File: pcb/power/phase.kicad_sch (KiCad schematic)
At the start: 9 parts, among them J1 Conn_01x02_Pin, J4 Conn_01x02_Pin, J7 Conn_01x02_Pin, Q10 IPT015N10NF2S, Q2 IPT015N10NF2S, Q5 IPT015N10NF2S, Q6 IPT015N10NF2S

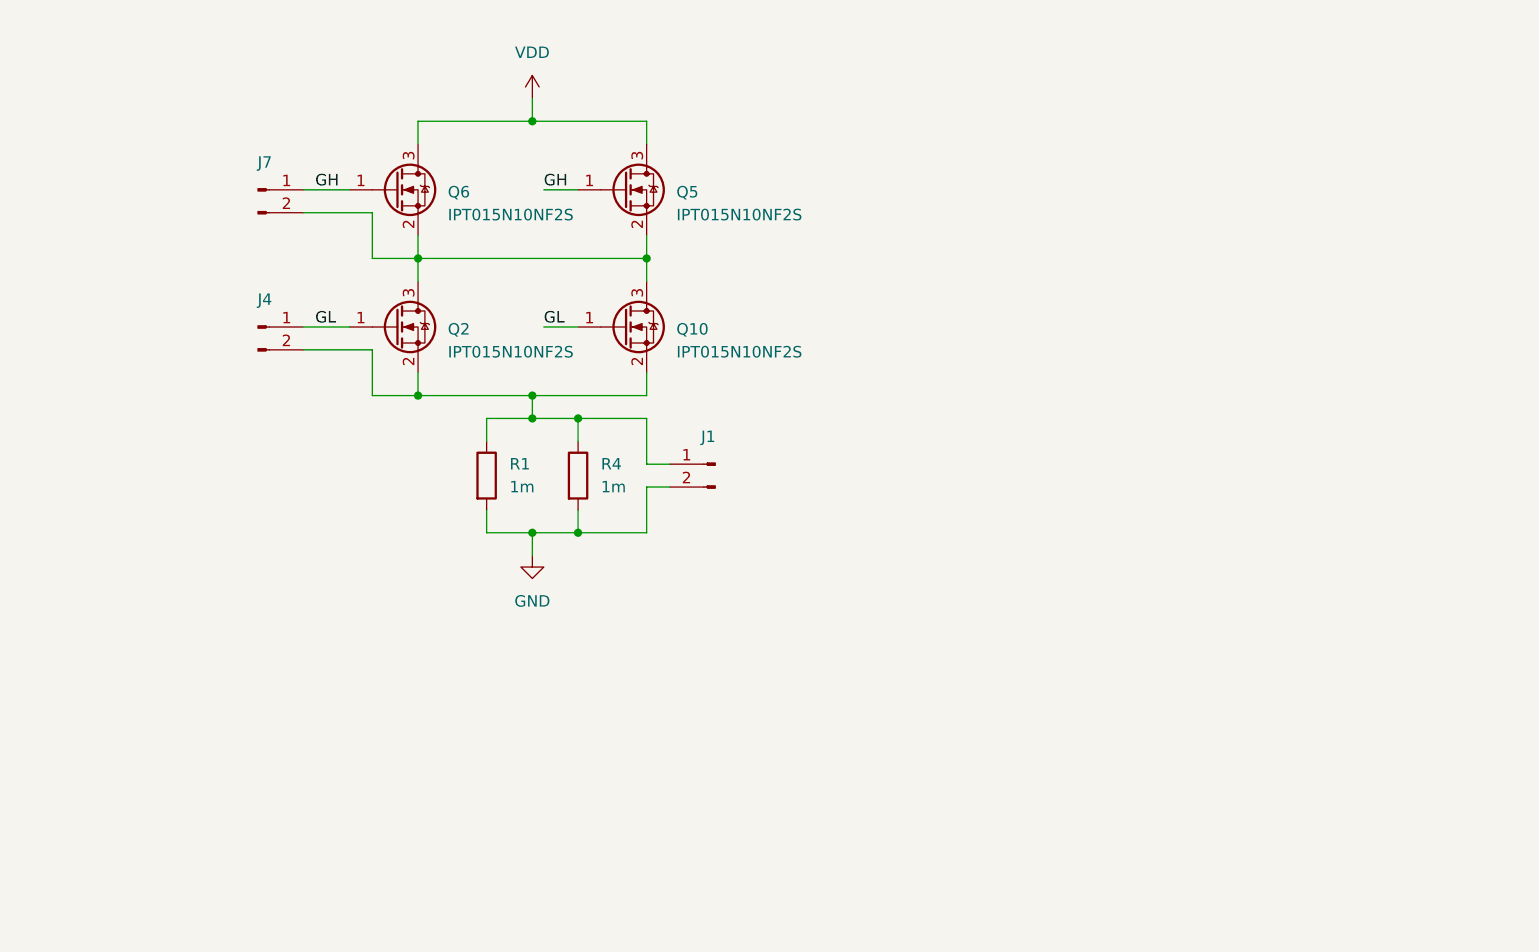
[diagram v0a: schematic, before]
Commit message: Semifinish power and bulk
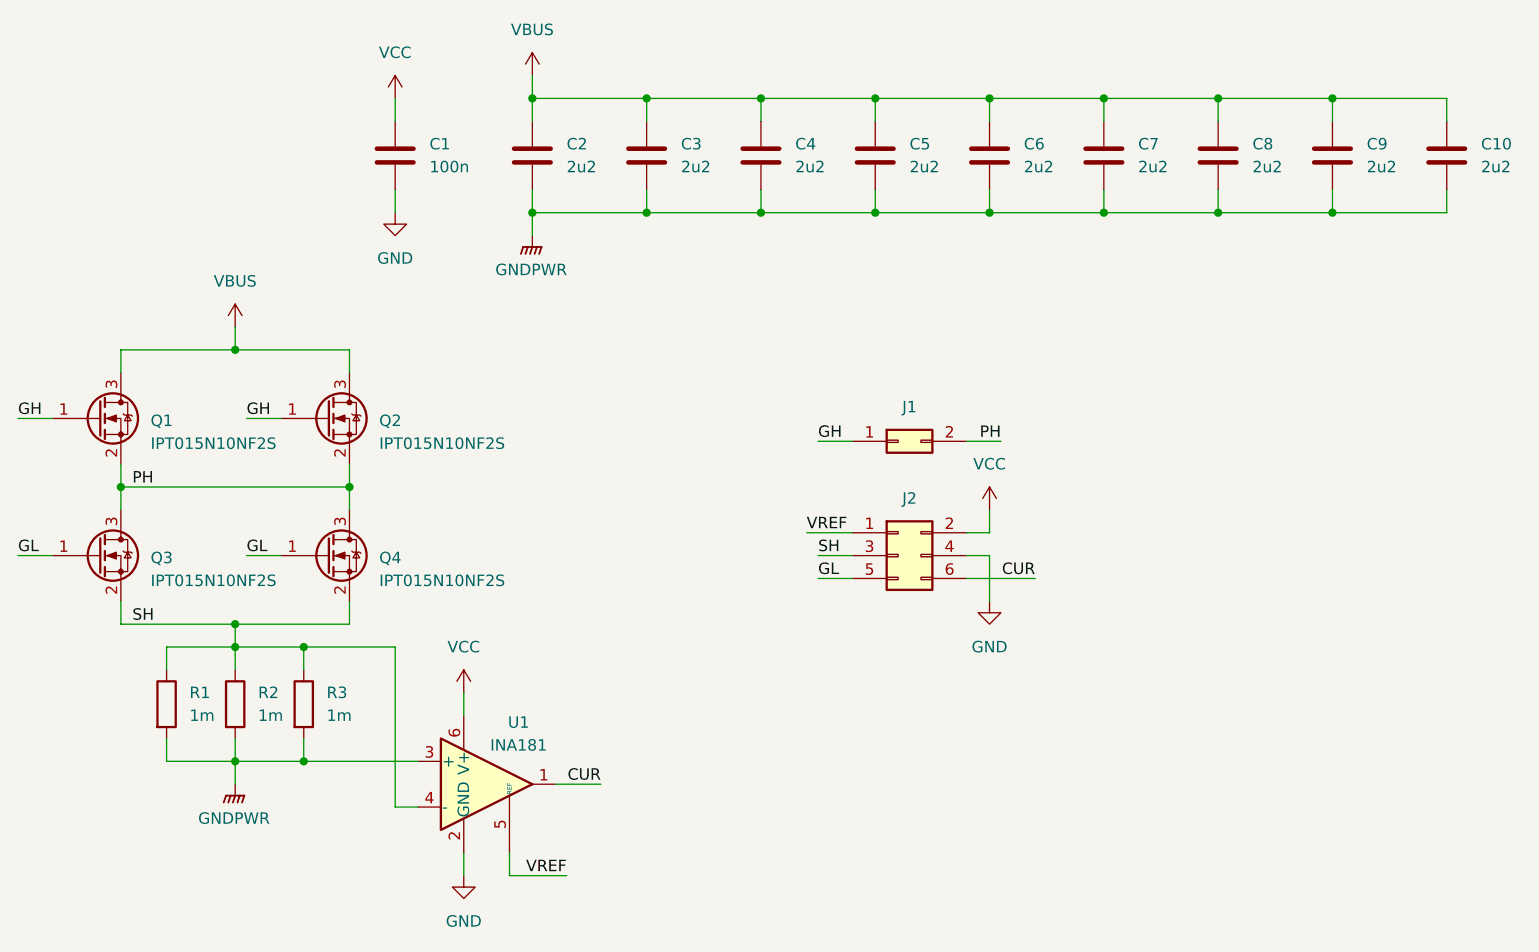
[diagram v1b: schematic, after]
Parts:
- removed J1, J4, J7: Conn_01x02_Pin, Connector_PinHeader_2.54mm:PinHeader_2x01_P2.54mm_Vertical_SMD, symbol Connector:Conn_01x02_Pin
- added C1: 100n, Capacitor_SMD:C_0402_1005Metric, symbol Device:C
- added C10, C2, C3, C4, C5, C6, C7, C8, C9: 2u2, Capacitor_SMD:C_1206_3216Metric, symbol Device:C
- added J1: Conn_02x01, Connector_PinHeader_1.27mm:PinHeader_2x01_P1.27mm_Vertical_SMD, symbol Connector_Generic:Conn_02x01
- added J2: Conn_02x03_Odd_Even, Connector_PinHeader_1.27mm:PinHeader_2x03_P1.27mm_Vertical_SMD, symbol Connector_Generic:Conn_02x03_Odd_Even
- added R2: 1m, Resistor_SMD:R_2512_6332Metric, symbol Device:R
- added U1: INA181, Package_TO_SOT_SMD:SOT-23-6, symbol Amplifier_Current:INA181
- R1: footprint Resistor_SMD:R_4020_10251Metric -> Resistor_SMD:R_2512_6332Metric; LCSC (none) -> C5123666
- R3: renamed from R4; footprint Resistor_SMD:R_4020_10251Metric -> Resistor_SMD:R_2512_6332Metric; LCSC (none) -> C5123666
- renumbered Q6 to Q1, Q5 to Q2, Q2 to Q3, Q10 to Q4
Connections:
- net GH: now also J1.1 (Pin_1)
- net GL: now also J2.5 (Pin_5)
- net GND: now also C1.2, J2.4 (Pin_4), U1.2 (GND); no longer R1.2, R3.2
- net SH: now reaches Q3.2 (S), Q4.2 (S), R1.1, R3.1
- net SH: now also J2.3 (Pin_3), R2.1, U1.4 (-)
- net PH: now reaches Q1.2 (S), Q2.2 (S), Q3.3 (D), Q4.3 (D)
- net PH: now also J1.2 (Pin_2)
- net VDD renamed VBUS
- net VBUS: now also C10.1, C2.1, C3.1, C4.1, C5.1, C6.1, C7.1, C8.1, C9.1
- new net CUR: J2.6 (Pin_6), U1.1
- new net GNDPWR: C10.2, C2.2, C3.2, C4.2, C5.2, C6.2, C7.2, C8.2, C9.2, R1.2, R2.2, R3.2, U1.3 (+)
- new net VCC: C1.1, J2.2 (Pin_2), U1.6 (V+)
- new net VREF: J2.1 (Pin_1), U1.5 (REF)
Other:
- moved on the sheet: Q1, Q2, Q3, Q4, R3
